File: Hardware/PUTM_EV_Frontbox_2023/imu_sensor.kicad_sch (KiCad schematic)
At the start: 4 parts, among them U17 IMS330DHCX

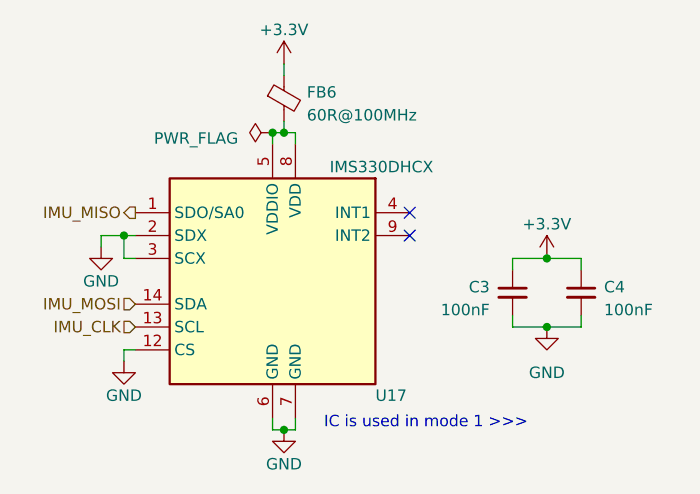
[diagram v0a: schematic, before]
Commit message: Grouped components
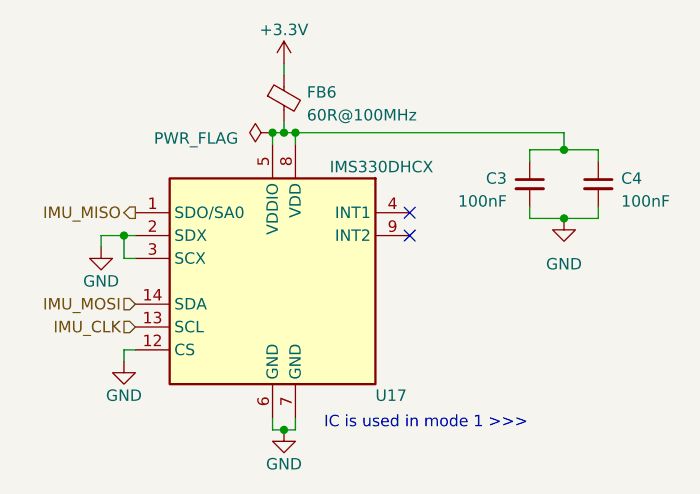
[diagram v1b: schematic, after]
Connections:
- net +3.3V: no longer C3.1, C4.1
- net at FB6.2, U17.5 (VDDIO), U17.8 (VDD): now also C3.1, C4.1
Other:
- moved on the sheet: C3, C4
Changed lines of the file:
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@@
   (junction (at 109.22 76.2) (diameter 0) (color 0 0 0 0)
   )
-  (junction (at 139.7 97.79) (diameter 0) (color 0 0 0 0)
+  (junction (at 141.605 85.725) (diameter 0) (color 0 0 0 0)
   )
   (junction (at 92.71 87.63) (diameter 0) (color 0 0 0 0)
   )
-  (junction (at 139.7 90.17) (diameter 0) (color 0 0 0 0)
+  (junction (at 141.605 78.105) (diameter 0) (color 0 0 0 0)
   )
   (junction (at 110.49 109.22) (diameter 0) (color 0 0 0 0)
   )
+  (junction (at 111.76 76.2) (diameter 0) (color 0 0 0 0)
+  )
   (junction (at 110.49 76.2) (diameter 0) (color 0 0 0 0)
   )
@@
     (stroke (width 0) (type default))
   )
-  (wire (pts (xy 143.51 91.44) (xy 143.51 90.17))
+  (wire (pts (xy 145.415 79.375) (xy 145.415 78.105))
+    (stroke (width 0) (type default))
+  )
+  (wire (pts (xy 111.76 76.2) (xy 141.605 76.2))
     (stroke (width 0) (type default))
   )
@@
     (stroke (width 0) (type default))
   )
-  (wire (pts (xy 143.51 90.17) (xy 139.7 90.17))
+  (wire (pts (xy 137.795 78.105) (xy 141.605 78.105))
     (stroke (width 0) (type default))
   )
@@
     (stroke (width 0) (type default))
   )
-  (wire (pts (xy 143.51 97.79) (xy 139.7 97.79))
+  (wire (pts (xy 145.415 85.725) (xy 141.605 85.725))
     (stroke (width 0) (type default))
   )
-  (wire (pts (xy 110.49 76.2) (xy 111.76 76.2))
+  (wire (pts (xy 109.22 109.22) (xy 110.49 109.22))
     (stroke (width 0) (type default))
   )
-  (wire (pts (xy 109.22 109.22) (xy 110.49 109.22))
+  (wire (pts (xy 141.605 76.2) (xy 141.605 78.105))
     (stroke (width 0) (type default))
   )
@@
     (stroke (width 0) (type default))
   )
-  (wire (pts (xy 135.89 91.44) (xy 135.89 90.17))
+  (wire (pts (xy 137.795 79.375) (xy 137.795 78.105))
     (stroke (width 0) (type default))
   )
-  (wire (pts (xy 135.89 96.52) (xy 135.89 97.79))
+  (wire (pts (xy 137.795 84.455) (xy 137.795 85.725))
     (stroke (width 0) (type default))
   )
-  (wire (pts (xy 135.89 90.17) (xy 139.7 90.17))
+  (wire (pts (xy 110.49 76.2) (xy 111.76 76.2))
     (stroke (width 0) (type default))
   )
@@
     (stroke (width 0) (type default))
   )
-  (wire (pts (xy 143.51 96.52) (xy 143.51 97.79))
+  (wire (pts (xy 145.415 84.455) (xy 145.415 85.725))
+    (stroke (width 0) (type default))
+  )
+  (wire (pts (xy 141.605 78.105) (xy 145.415 78.105))
     (stroke (width 0) (type default))
   )
@@
     (stroke (width 0) (type default))
   )
-  (wire (pts (xy 135.89 97.79) (xy 139.7 97.79))
+  (wire (pts (xy 137.795 85.725) (xy 141.605 85.725))
     (stroke (width 0) (type default))
   )
@@
     )
   )
-  (symbol (lib_id "power:GND") (at 139.7 97.79 0) (unit 1)
+  (symbol (lib_id "power:GND") (at 141.605 85.725 0) (unit 1)
     (in_bom yes) (on_board yes) (dnp no) (fields_autoplaced)
-    (property "Reference" "#PWR032" (at 139.7 104.14 0)
+    (property "Reference" "#PWR032" (at 141.605 92.075 0)
       (effects (font (size 1.27 1.27)) hide)
     )
-    (property "Value" "GND" (at 139.7 102.87 0)
+    (property "Value" "GND" (at 141.605 90.805 0)
       (effects (font (size 1.27 1.27)))
     )
-    (property "Footprint" "" (at 139.7 97.79 0)
+    (property "Footprint" "" (at 141.605 85.725 0)
       (effects (font (size 1.27 1.27)) hide)
     )
-    (property "Datasheet" "" (at 139.7 97.79 0)
+    (property "Datasheet" "" (at 141.605 85.725 0)
       (effects (font (size 1.27 1.27)) hide)
     )
@@
     )
   )
-  (symbol (lib_id "power:+3.3V") (at 139.7 90.17 0) (unit 1)
-    (in_bom yes) (on_board yes) (dnp no) (fields_autoplaced)
-    (property "Reference" "#PWR031" (at 139.7 93.98 0)
-      (effects (font (size 1.27 1.27)) hide)
-    )
-    (property "Value" "+3.3V" (at 139.7 86.36 0)
-      (effects (font (size 1.27 1.27)))
-    )
-    (property "Footprint" "" (at 139.7 90.17 0)
-      (effects (font (size 1.27 1.27)) hide)
-    )
-    (property "Datasheet" "" (at 139.7 90.17 0)
-      (effects (font (size 1.27 1.27)) hide)
-    )
-    (pin "1")
-    (instances
-      (project "PUTM_EV_Frontbox_2023"
-        (path "/b652b05a-4e3d-4ad1-b032-18886abe7d45/fc1ffdcd-7b51-43f2-87c4-9a5d8609cd78"
-          (reference "#PWR031") (unit 1)
-        )
-      )
-    )
-  )
-  (symbol (lib_id "Device:C_Small") (at 135.89 93.98 0) (mirror y) (unit 1)
+  (symbol (lib_id "Device:C_Small") (at 137.795 81.915 0) (mirror y) (unit 1)
     (in_bom yes) (on_board yes) (dnp no)
-    (property "Reference" "C3" (at 133.35 93.3513 0)
+    (property "Reference" "C3" (at 135.255 81.2863 0)
       (effects (font (size 1.27 1.27)) (justify left))
     )
-    (property "Value" "100nF" (at 133.35 95.8913 0)
+    (property "Value" "100nF" (at 135.255 83.8263 0)
       (effects (font (size 1.27 1.27)) (justify left))
     )
-    (property "Footprint" "Capacitor_SMD:C_0402_1005Metric_Pad0.74x0.62mm_HandSolder" (at 135.89 93.98 0)
+    (property "Footprint" "Capacitor_SMD:C_0402_1005Metric_Pad0.74x0.62mm_HandSolder" (at 137.795 81.915 0)
       (effects (font (size 1.27 1.27)) hide)
     )
-    (property "Datasheet" "~" (at 135.89 93.98 0)
+    (property "Datasheet" "~" (at 137.795 81.915 0)
       (effects (font (size 1.27 1.27)) hide)
     )
@@
     )
   )
-  (symbol (lib_id "Device:C_Small") (at 143.51 93.98 0) (unit 1)
+  (symbol (lib_id "Device:C_Small") (at 145.415 81.915 0) (unit 1)
     (in_bom yes) (on_board yes) (dnp no)
-    (property "Reference" "C4" (at 146.05 93.3513 0)
+    (property "Reference" "C4" (at 147.955 81.2863 0)
       (effects (font (size 1.27 1.27)) (justify left))
     )
-    (property "Value" "100nF" (at 146.05 95.8913 0)
+    (property "Value" "100nF" (at 147.955 83.8263 0)
       (effects (font (size 1.27 1.27)) (justify left))
     )
-    (property "Footprint" "Capacitor_SMD:C_0402_1005Metric_Pad0.74x0.62mm_HandSolder" (at 143.51 93.98 0)
+    (property "Footprint" "Capacitor_SMD:C_0402_1005Metric_Pad0.74x0.62mm_HandSolder" (at 145.415 81.915 0)
       (effects (font (size 1.27 1.27)) hide)
     )
-    (property "Datasheet" "~" (at 143.51 93.98 0)
+    (property "Datasheet" "~" (at 145.415 81.915 0)
       (effects (font (size 1.27 1.27)) hide)
     )
